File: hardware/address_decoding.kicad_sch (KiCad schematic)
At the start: 9 parts, among them U2 74HC30, U3 74AHC00, U4 74AHC32, U5 74AHC138

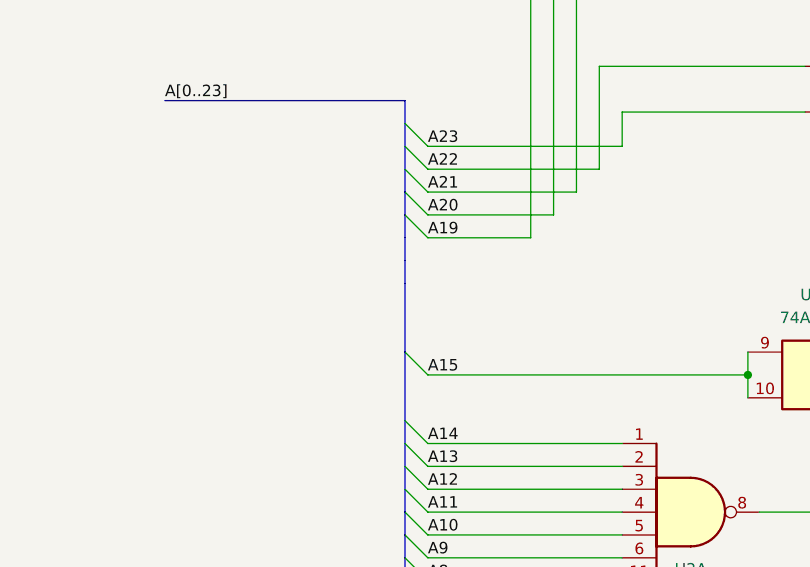
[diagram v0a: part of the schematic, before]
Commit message: CLeanup
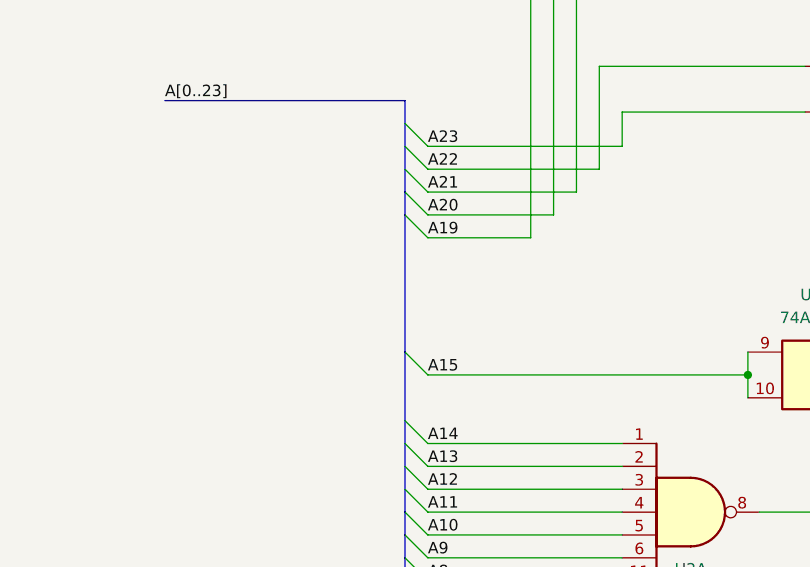
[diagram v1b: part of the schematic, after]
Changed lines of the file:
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@@
-    (stroke (width 0) (type default) (color 0 0 0 0))
-  )
-  (bus (pts (xy 120.65 80.01) (xy 120.65 87.63))
     (stroke (width 0) (type default) (color 0 0 0 0))
   )
@@
     (stroke (width 0) (type default) (color 0 0 0 0))
   )
-  (bus (pts (xy 120.65 74.93) (xy 120.65 77.47))
+  (bus (pts (xy 120.65 72.39) (xy 120.65 87.63))
     (stroke (width 0) (type default) (color 0 0 0 0))
   )
@@
     (stroke (width 0) (type default) (color 0 0 0 0))
   )
-  (bus (pts (xy 120.65 72.39) (xy 120.65 74.93))
-    (stroke (width 0) (type default) (color 0 0 0 0))
-  )
   (wire (pts (xy 205.74 50.8) (xy 205.74 45.72))
     (stroke (width 0) (type default) (color 0 0 0 0))
@@
     (stroke (width 0) (type default) (color 0 0 0 0))
   )
-  (bus (pts (xy 120.65 77.47) (xy 120.65 80.01))
-    (stroke (width 0) (type default) (color 0 0 0 0))
-  )
